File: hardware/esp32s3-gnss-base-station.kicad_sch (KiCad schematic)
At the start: 9 parts, among them SW1 SS-12D10L5

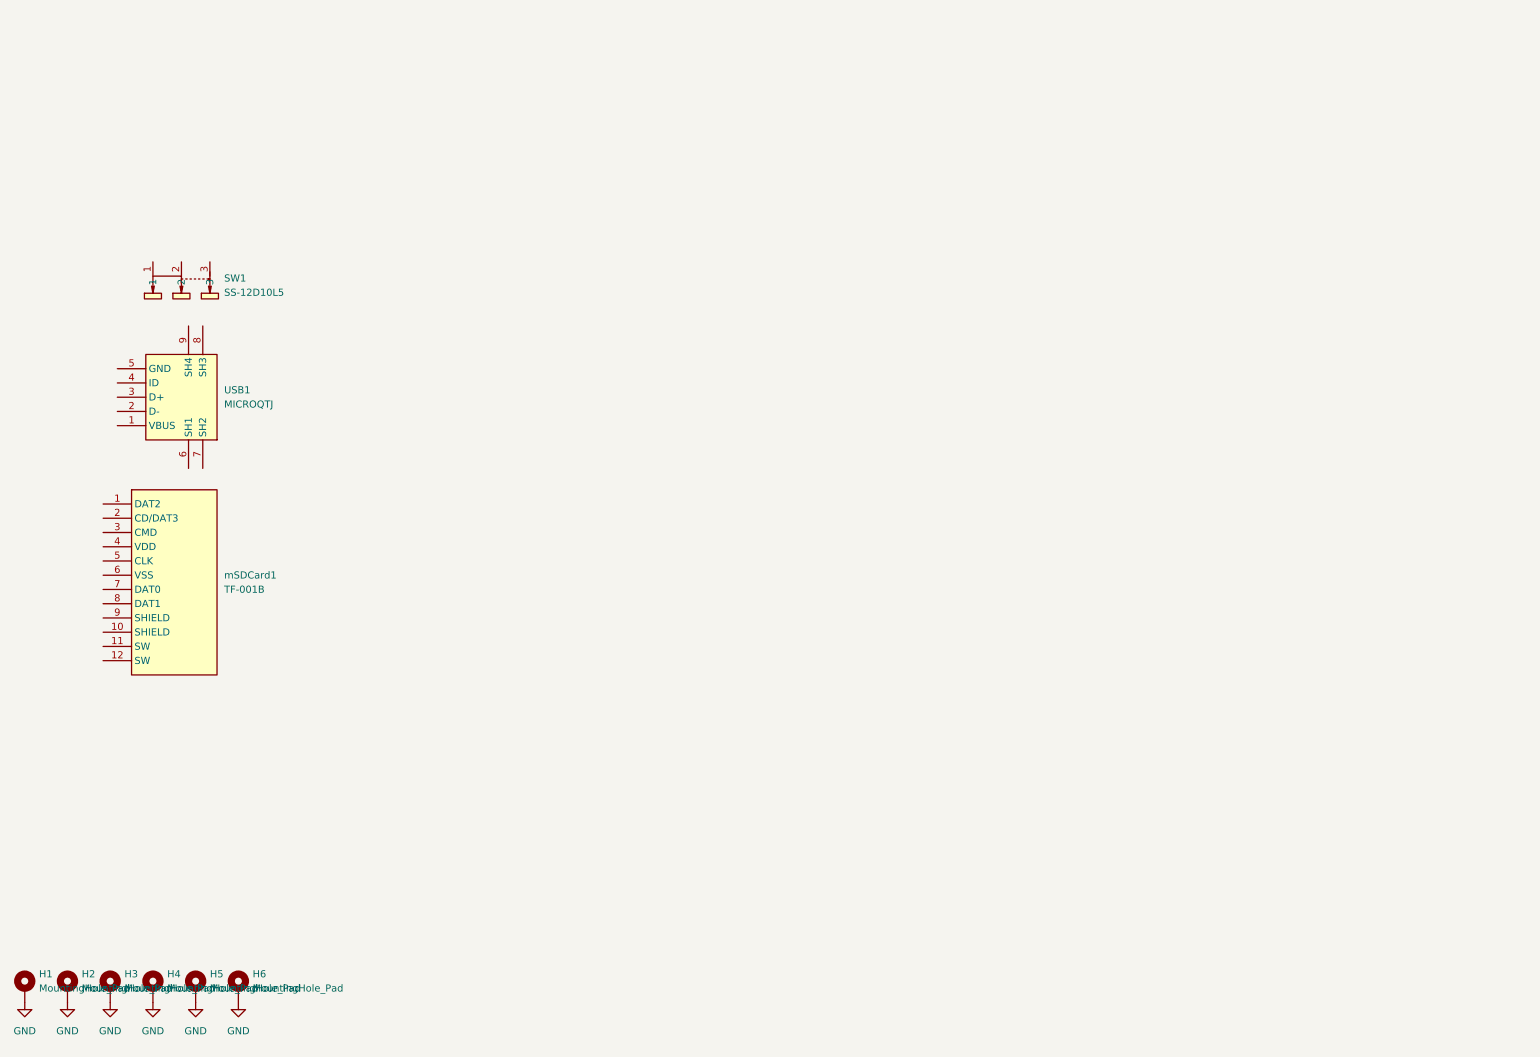
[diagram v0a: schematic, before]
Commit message: Add KiCAD Schematic v0.1
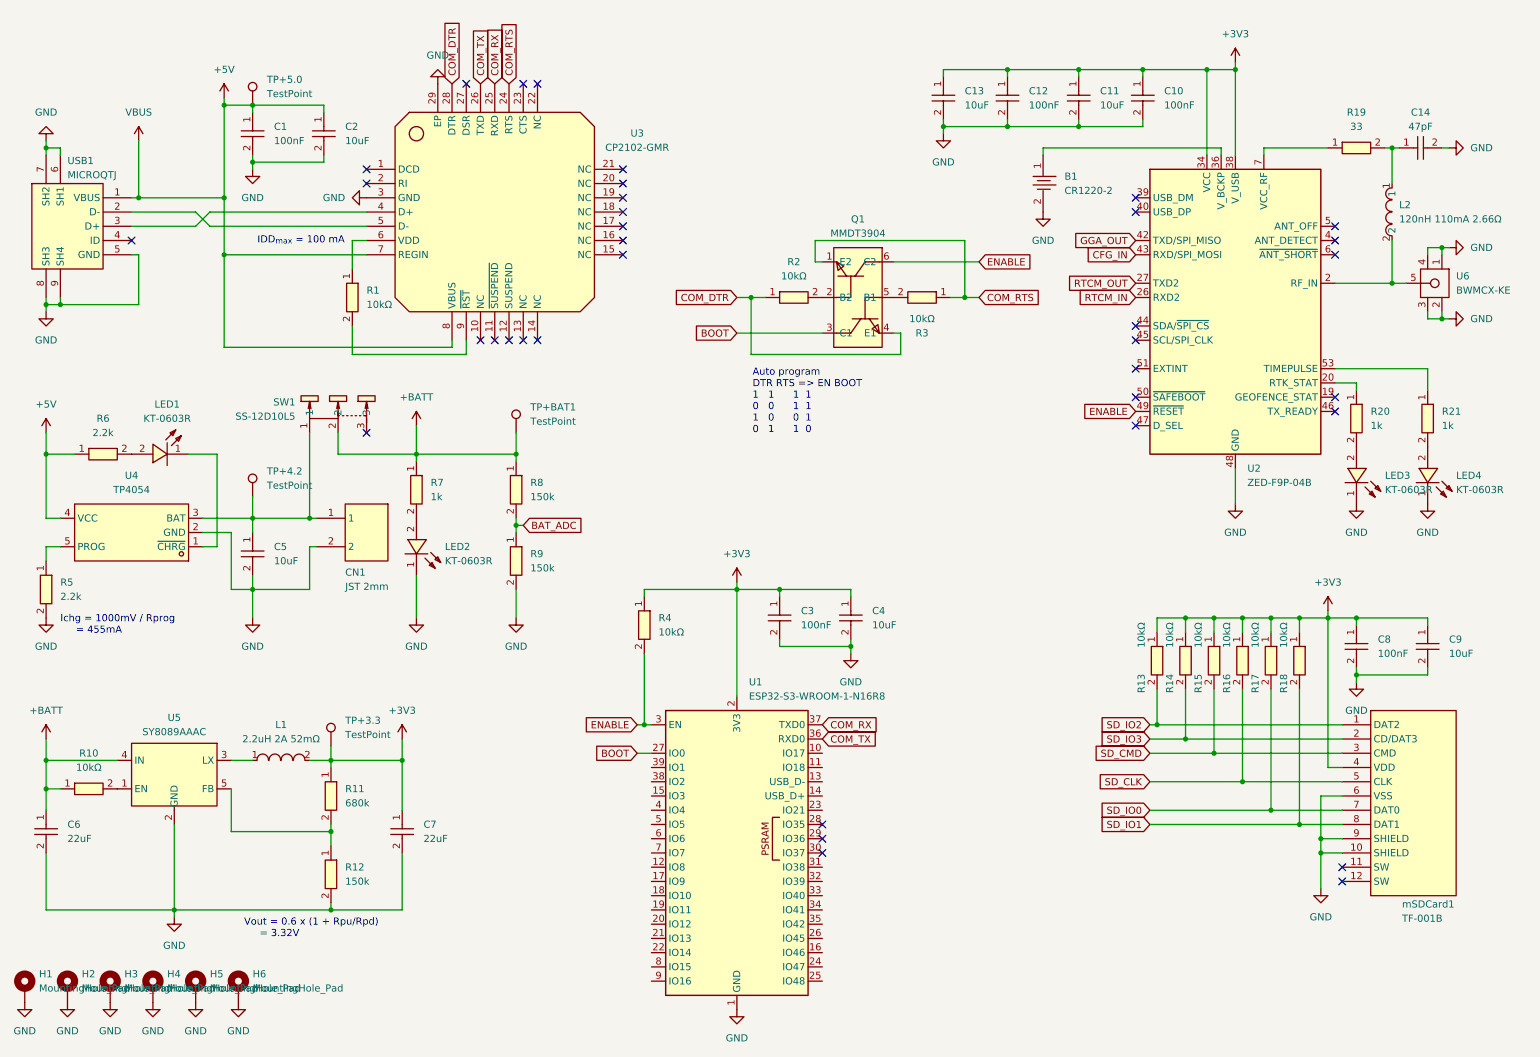
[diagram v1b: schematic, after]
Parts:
- added B1: CR1220-2, LCSC:BAT-SMD_CR1220-2, symbol LCSC:CR1220-2
- added C1, C10, C12, C3, C8: 100nF, LCSC:C0402, symbol LCSC:CL05B104KO5NNNC
- added C11, C13, C2, C4, C5, C9: 10uF, LCSC:C0603, symbol LCSC:CL10A106MA8NRNC
- added C14: 47pF, LCSC:C0603, symbol LCSC:CL10C470JB8NNNC
- added C6, C7: 22uF, LCSC:C0805, symbol LCSC:CL21A226MAQNNNE
- added CN1: JST 2mm, LCSC:CONN-TH_B2B-PH-K-S, symbol LCSC:B2B-PH-K-S(LF)(SN)
- added L1: 2.2uH 2A 52mΩ, LCSC:IND-SMD_L4.0-W4.0, symbol LCSC:SWPA4026S2R2MT
- added L2: 120nH 110mA 2.66Ω, LCSC:L0402, symbol LCSC:LQW15ANR12J00D
- added LED1, LED2, LED3, LED4: KT-0603R, LCSC:LED0603-RD, symbol LCSC:KT-0603R
- added Q1: MMDT3904, LCSC:SOT-363_L2.0-W1.3-P0.65-LS2.1-BR, symbol LCSC:MMDT3904
- added R1, R10, R13, R14, R15, R16, R17, R18, R2, R3, R4: 10kΩ, LCSC:R0603, symbol LCSC:0603WAF1002T5E
- added R11: 680k, LCSC:R0603, symbol LCSC:0603WAF6803T5E
- added R12, R8, R9: 150k, LCSC:R0603, symbol LCSC:0603WAF1503T5E
- added R19: 33, LCSC:R0603, symbol LCSC:0603WAF330JT5E
- added R20, R21, R7: 1k, LCSC:R0603, symbol LCSC:0603WAF1001T5E
- added R5, R6: 2.2k, LCSC:R0603, symbol LCSC:0603WAF2201T5E
- added TP+3.3, TP+4.2, TP+5.0, TP+BAT1: TestPoint, TestPoint:TestPoint_Pad_D1.5mm, symbol Connector:TestPoint
- added U1: ESP32-S3-WROOM-1-N16R8, RF_Module:ESP32-S3-WROOM-1, symbol RF_Module:ESP32-S3-WROOM-1
- added U2: ZED-F9P-04B, RF_GPS:ublox_ZED, symbol RF_GPS:ZED-F9P
- added U3: CP2102-GMR, LCSC:WQFN-28_L5.0-W5.0-P0.50-BL-EP3.2, symbol LCSC:CP2102-GMR
- added U4: TP4054, LCSC:SOT-23-5_L3.0-W1.7-P0.95-LS2.8-BL, symbol LCSC:TP4054
- added U5: SY8089AAAC, LCSC:SOT-23-5_L3.0-W1.7-P0.95-LS2.8-BR, symbol LCSC:SY8089AAAC
- added U6: BWMCX-KE, LCSC:SMA-TH_BWMCX-KE, symbol LCSC:BWMCX-KE
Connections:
- net GND: now also USB1.5 (GND), USB1.6 (SH1), USB1.7 (SH2), USB1.8 (SH3), USB1.9 (SH4), mSDCard1.10 (SHIELD), mSDCard1.6 (VSS), mSDCard1.9 (SHIELD), B1.2, C1.2, C10.2, C11.2, C12.2, C13.2, C14.2, C2.2, C3.2, C4.2, C5.2, C6.2, C7.2, C8.2, C9.2, CN1.2, LED2.1, LED3.1, LED4.1, R12.2, R5.2, R9.2, U1.1 (GND), U1.40 (GND), U1.41 (GND), U2.1 (GND), U2.12 (GND), U2.14 (GND), U2.3 (GND), U2.32 (GND), U2.37 (GND), U2.41 (GND), U2.48 (GND), U2.55 (GND), U3.29 (EP), U3.3 (GND), U4.2 (GND), U5.2 (GND), U6.1, U6.2, U6.3, U6.4
- net +5V: now reaches USB1.1 (VBUS)
- net +5V: now also C1.1, C2.1, R6.1, TP+5.0.1, U3.7 (REGIN), U3.8 (VBUS), U4.4 (VCC)
- net at USB1.2 (D-): now also U3.5 (D-)
- net at USB1.3 (D+): now also U3.4 (D+)
- net at SW1.1: now also C5.1, CN1.1, TP+4.2.1, U4.3 (BAT)
- net +BATT: now reaches SW1.2
- net +BATT: now also C6.1, R10.1, R7.1, R8.1, TP+BAT1.1, U5.4 (IN)
- net SD_IO2: now reaches mSDCard1.1 (DAT2)
- net SD_IO2: now also R13.2
- net SD_IO3: now reaches mSDCard1.2 (CD/DAT3)
- net SD_IO3: now also R14.2
- net SD_CMD: now reaches mSDCard1.3 (CMD)
- net SD_CMD: now also R15.2
- net +3V3: now reaches mSDCard1.4 (VDD)
- net +3V3: now also C10.1, C11.1, C12.1, C13.1, C3.1, C4.1, C7.1, C8.1, C9.1, L1.2, R11.1, R13.1, R14.1, R15.1, R16.1, R17.1, R18.1, R4.1, TP+3.3.1, U1.2 (3V3), U2.33 (VCC), U2.34 (VCC), U2.38 (V_USB)
- net SD_CLK: now reaches mSDCard1.5 (CLK)
- net SD_CLK: now also R16.2
- net SD_IO0: now reaches mSDCard1.7 (DAT0)
- net SD_IO0: now also R17.2
- net SD_IO1: now reaches mSDCard1.8 (DAT1)
- net SD_IO1: now also R18.2
- new net: R11.2, R12.1, U5.5 (FB)
- new net: Q1.2 (B2), R2.2
- new net: R1.1, U3.6 (VDD)
- new net: R1.2, U3.9 (~{RST})
- new net: R21.1, U2.53 (TIMEPULSE)
- new net: LED4.2, R21.2
- new net: R20.1, U2.20 (RTK_STAT)
- new net: LED3.2, R20.2
- new net: L1.1, U5.3 (LX)
- new net: L2.2, U2.2 (RF_IN), U6.5
- new net: B1.1, U2.36 (V_BCKP)
- new net: R19.1, U2.7 (VCC_RF)
- new net: C14.1, L2.1, R19.2
- new net: Q1.5 (B1), R3.2
- new net: R10.2, U5.1 (EN)
- new net: LED2.2, R7.2
- new net: LED1.2, R6.2
- new net: LED1.1, U4.1 (~{CHRG})
- new net: R5.1, U4.5 (PROG)
- new net BAT_ADC: R8.2, R9.1
- new net BOOT: Q1.3 (C1), U1.27 (IO0)
- new net CFG_IN: U2.43 (RXD/SPI_MOSI)
- new net COM_DTR: Q1.4 (E1), R2.1, U3.28 (DTR)
- new net COM_RTS: Q1.1 (E2), R3.1, U3.24 (RTS)
- new net COM_RX: U1.37 (TXD0), U3.25 (RXD)
- new net COM_TX: U1.36 (RXD0), U3.26 (TXD)
- new net ENABLE: Q1.6 (C2), R4.2, U1.3 (EN), U2.49 (~{RESET})
- new net GGA_OUT: U2.42 (TXD/SPI_MISO)
- new net RTCM_IN: U2.26 (RXD2)
- new net RTCM_OUT: U2.27 (TXD2)
- no-connect marks 0 -> 36
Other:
- note added: "Auto program DTR RTS => EN BOOT 1 1 1 1 0 0 1 1 1 0 0 1 0 1 1 0"
- note added: "IDD_{max} = 100 mA"
- note added: "Ichg = 1000mV / Rprog = 455mA"
- note added: "Vout = 0.6 x (1 + Rpu/Rpd) = 3.32V"
- moved on the sheet: SW1, USB1, mSDCard1
